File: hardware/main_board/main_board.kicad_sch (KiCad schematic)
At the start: 15 parts, among them J1 Conn_01x01_Pin, J2 Conn_01x02_Pin, J3 Conn_02x12_Odd_Even, J4 Conn_02x12_Odd_Even, J5 SJ3-35083C-TR, J6 SJ3-35083C-TR, J7 Barrel_Jack_Switch_Pin3Ring, U1 CD40109BE, U2 L78M05CV

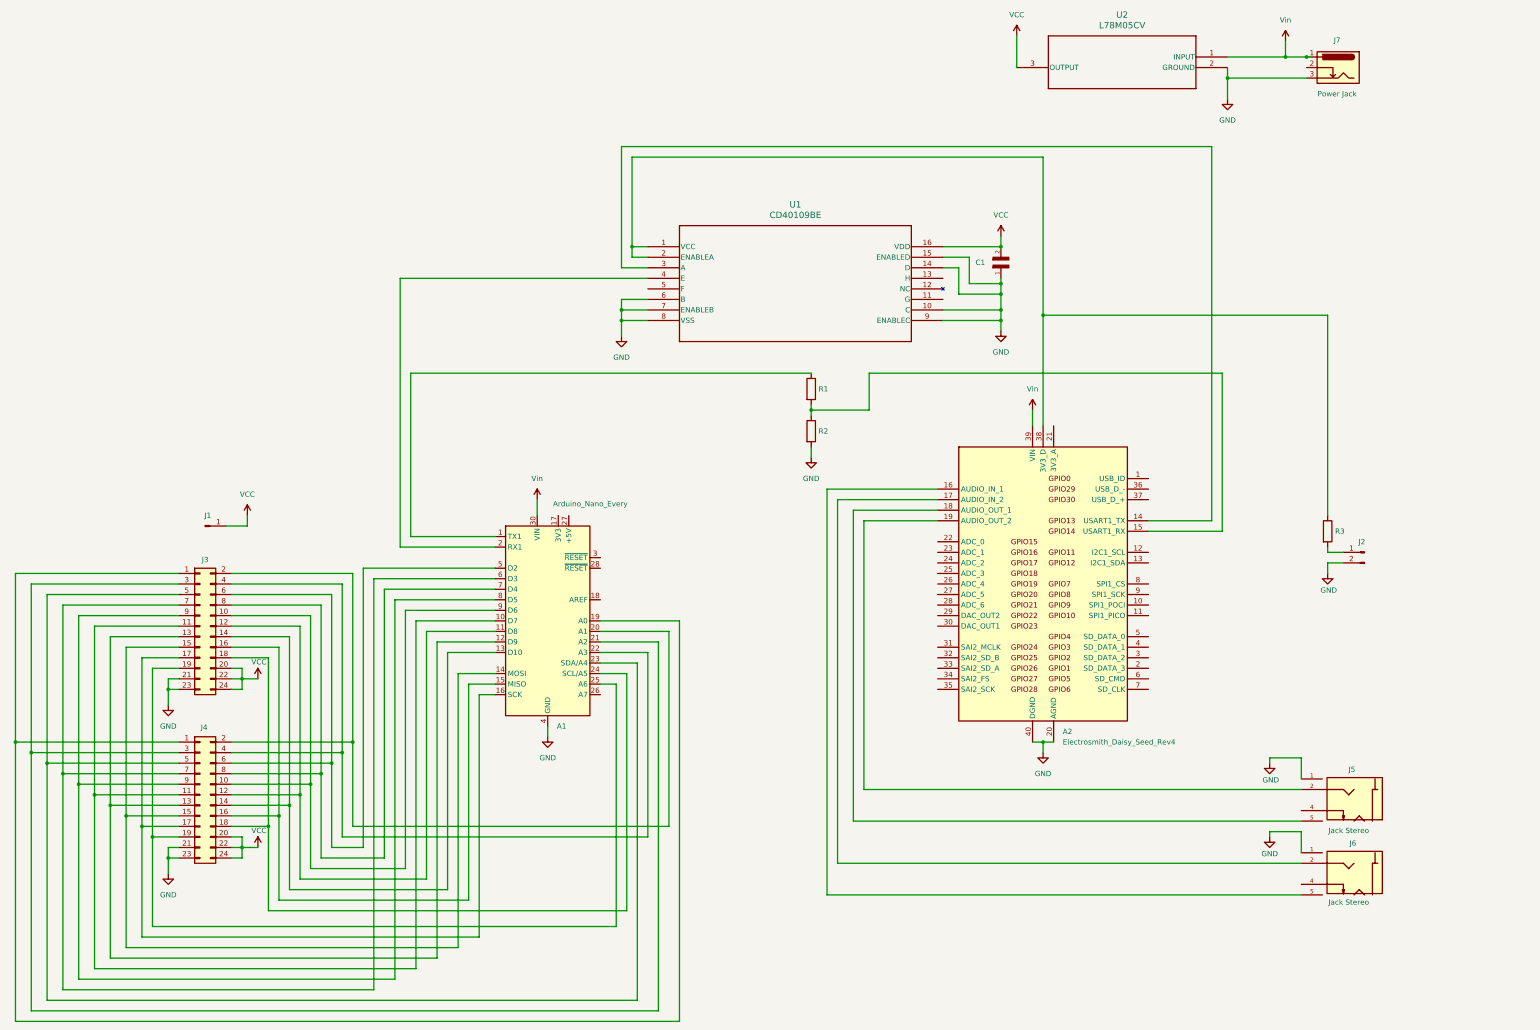
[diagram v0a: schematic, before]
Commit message: First test passed with main boards and all satellite boards connected
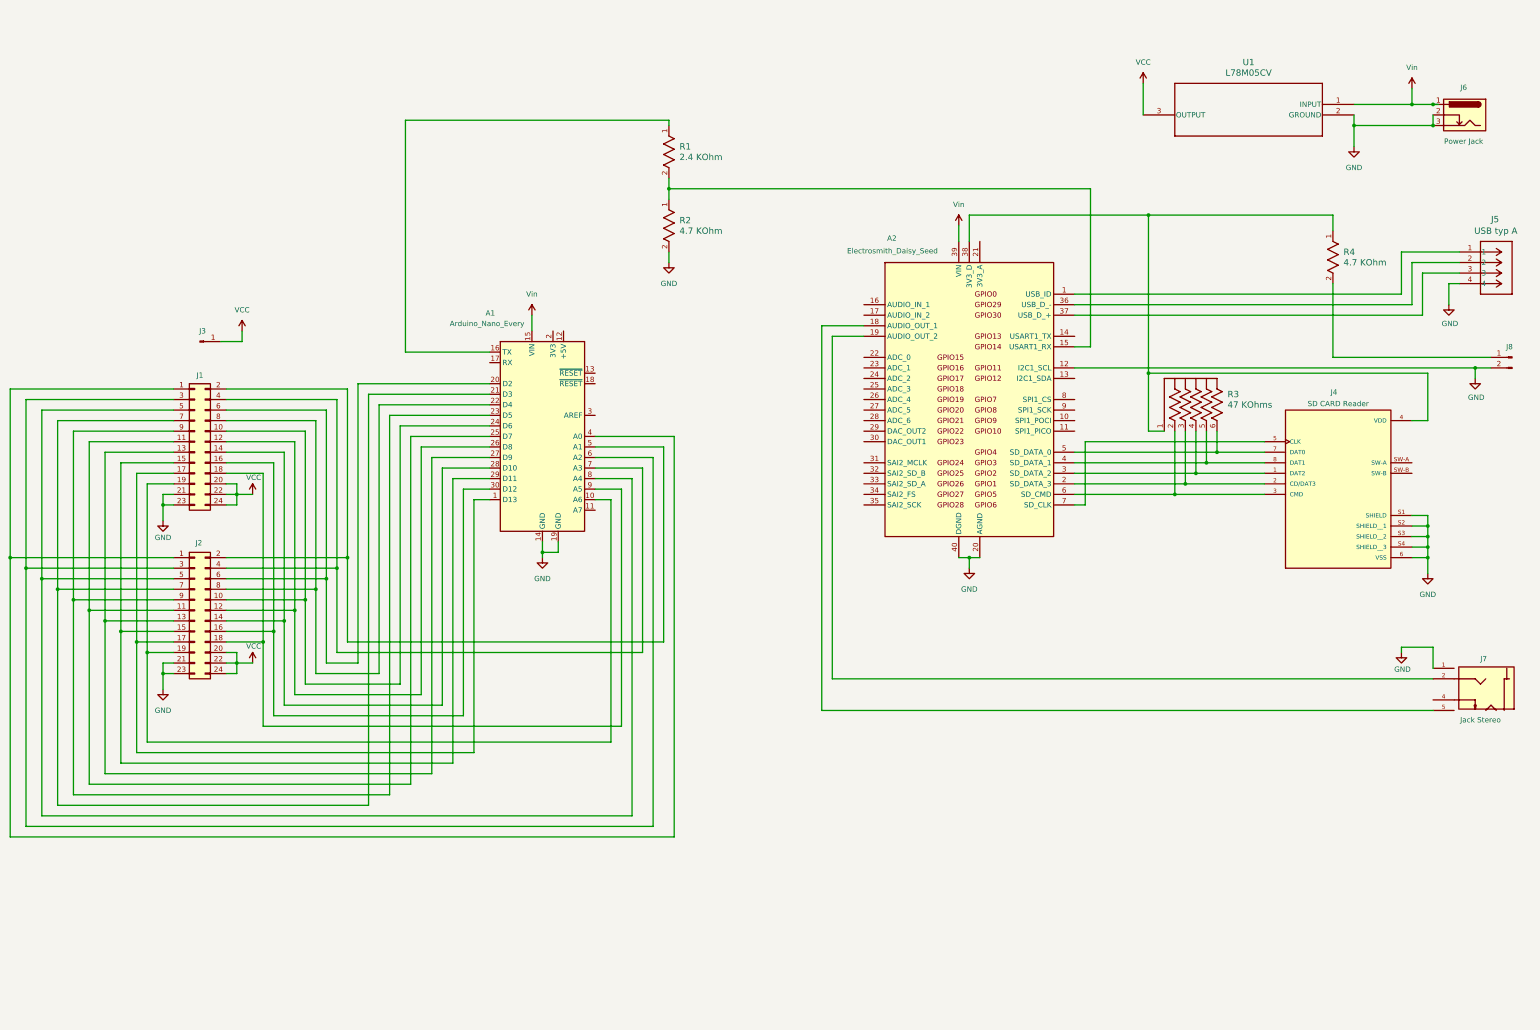
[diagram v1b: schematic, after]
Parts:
- removed C1: B32529C0102K289, B32529C0102K289:CAPRR500W50L730T250H650, symbol B32529C0102K289:B32529C0102K289
- removed J6: SJ3-35083C-TR, SJ3_35083C_TR:SAMESKY_SJ3-35083C-TR, symbol SJ3-35083C-TR:SJ3-35083C-TR
- removed R1, R2, R3: R, symbol Device:R
- removed U1: CD40109BE, CD40109BE:N16, symbol 2024-12-24_11-42-04:CD40109BE
- added J4: SD CARD Reader, DM3D_SF:HRS_DM3D-SF, symbol DM3D-SF:DM3D-SF
- added J5: USB typ A, 676433910:CONN_67643-3910_MOL, symbol 676433910:676433910
- added R1: 2.4 KOhm, CF14JT4K70:STA_CF14_STP, symbol CF14JT4K70:CF14JT4K70
- added R2, R4: 4.7 KOhm, CF14JT4K70:STA_CF14_STP, symbol CF14JT4K70:CF14JT4K70
- added R3: 47 KOhms, 4606X_101_473LF:BO_4606X, symbol 2025-01-10_20-55-13:4606X-101-473LF
- A2: value Electrosmith_Daisy_Seed_Rev4 -> Electrosmith_Daisy_Seed
- renumbered J3 to J1, J4 to J2, J1 to J3, J7 to J6, J5 to J7, J2 to J8, U2 to U1
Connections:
- net GND: now also A1.14 (GND), A1.19 (GND), A2.12 (I2C1_SCL), J6.2, J4.6 (VSS), J4.S1 (SHIELD), J4.S2 (SHIELD__1), J4.S3 (SHIELD__2), J4.S4 (SHIELD__3), J5.4, R2.2; no longer A1.29 (GND), A1.4 (GND)
- net Vin: now also A1.15 (VIN); no longer A1.30 (VIN)
- net at A2.38 (3V3_D): now also J4.4 (VDD), R3.1, R4.1
- net at J1.1 (Pin_1), J2.1 (Pin_1): now also A1.4 (A0); no longer A1.19 (A0)
- net at J1.10 (Pin_10), J2.10 (Pin_10): now also A1.24 (D6); no longer A1.9 (D6)
- net at J1.11 (Pin_11), J2.11 (Pin_11): now also A1.25 (D7); no longer A1.10 (D7)
- net at J1.12 (Pin_12), J2.12 (Pin_12): now also A1.26 (D8); no longer A1.11 (D8)
- net at J1.13 (Pin_13), J2.13 (Pin_13): now also A1.27 (D9); no longer A1.12 (D9)
- net at J1.14 (Pin_14), J2.14 (Pin_14): now also A1.28 (D10); no longer A1.13 (D10)
- net at J1.15 (Pin_15), J2.15 (Pin_15): now also A1.29 (D11); no longer A1.14 (MOSI)
- net at J1.16 (Pin_16), J2.16 (Pin_16): now also A1.30 (D12); no longer A1.15 (MISO)
- net at J1.17 (Pin_17), J2.17 (Pin_17): now also A1.1 (D13); no longer A1.16 (SCK)
- net at J1.18 (Pin_18), J2.18 (Pin_18): now also A1.9 (A5); no longer A1.24 (SCL/A5)
- net at J1.19 (Pin_19), J2.19 (Pin_19): now also A1.10 (A6); no longer A1.25 (A6)
- net at J1.2 (Pin_2), J2.2 (Pin_2): now also A1.5 (A1); no longer A1.20 (A1)
- net at J1.3 (Pin_3), J2.3 (Pin_3): now also A1.6 (A2); no longer A1.21 (A2)
- net at J1.4 (Pin_4), J2.4 (Pin_4): now also A1.7 (A3); no longer A1.22 (A3)
- net at J1.5 (Pin_5), J2.5 (Pin_5): now also A1.8 (A4); no longer A1.23 (SDA/A4)
- net at J1.6 (Pin_6), J2.6 (Pin_6): now also A1.20 (D2); no longer A1.5 (D2)
- net at J1.7 (Pin_7), J2.7 (Pin_7): now also A1.21 (D3); no longer A1.6 (D3)
- net at J1.8 (Pin_8), J2.8 (Pin_8): now also A1.22 (D4); no longer A1.7 (D4)
- net at J1.9 (Pin_9), J2.9 (Pin_9): now also A1.23 (D5); no longer A1.8 (D5)
- net at J8.1 (Pin_1): now also R4.2
- net at A2.15 (USART1_RX): now also R1.2, R2.1
- net at A2.1 (USB_ID): now also J5.1
- net at A2.2 (SD_DATA_3): now also J4.2 (CD/DAT3), R3.3
- net at A2.3 (SD_DATA_2): now also J4.1 (DAT2), R3.4
- net at A2.36 (USB_D_-): now also J5.2
- net at A2.37 (USB_D_+): now also J5.3
- net at A2.4 (SD_DATA_1): now also J4.8 (DAT1), R3.5
- net at A2.5 (SD_DATA_0): now also J4.7 (DAT0), R3.6
- net at A2.6 (SD_CMD): now also J4.3 (CMD), R3.2
- net at A2.7 (SD_CLK): now also J4.5 (CLK)
- new net: A1.16 (TX), R1.1
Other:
- moved on the sheet: A2, J1, J2, J3, J6, J7, J8, U1
